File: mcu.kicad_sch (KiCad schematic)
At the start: 46 parts, among them CN100 HX JN1.27-2X5 TP H4.9, J100 DM3CS-SF, U100 SW_RUN, U101 STM32F405RGTx, X100 X1E000210127000G

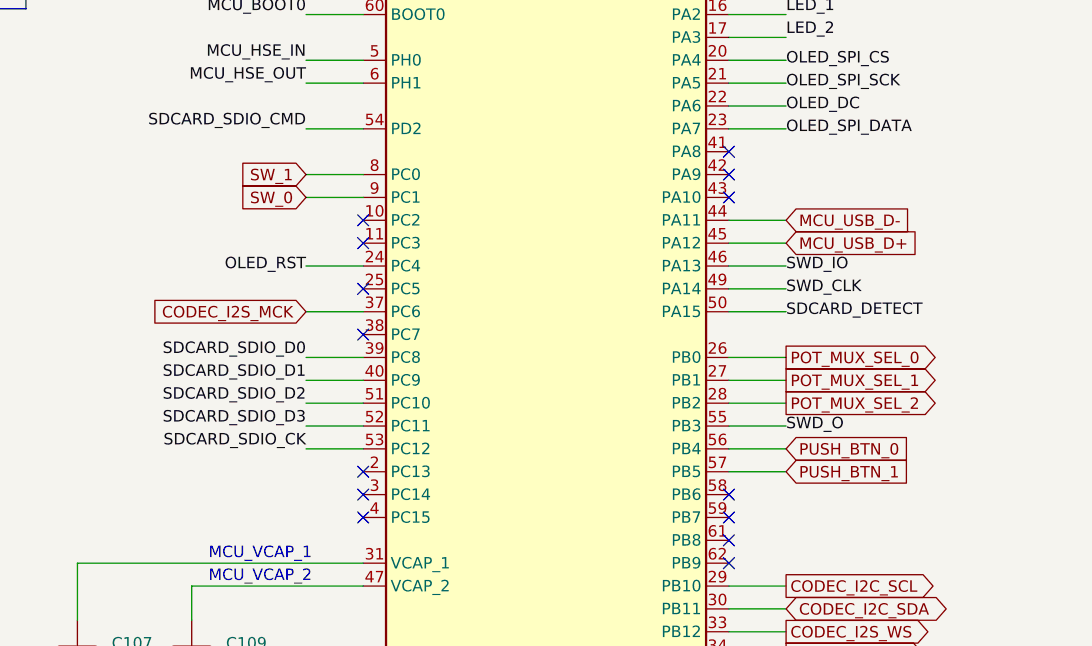
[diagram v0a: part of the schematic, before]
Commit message: last status
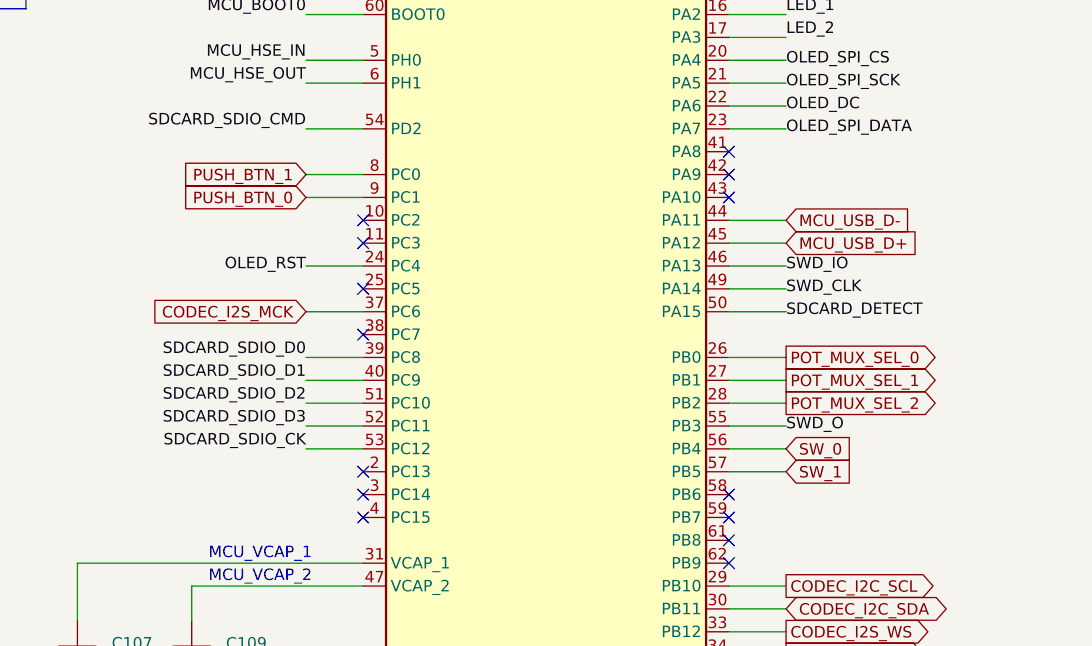
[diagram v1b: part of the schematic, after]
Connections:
- net PUSH_BTN_0: now also U101.9 (PC1); no longer U101.56 (PB4)
- net PUSH_BTN_1: now also U101.8 (PC0); no longer U101.57 (PB5)
- net SW_0: now also U101.56 (PB4); no longer U101.9 (PC1)
- net SW_1: now also U101.57 (PB5); no longer U101.8 (PC0)
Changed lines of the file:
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@@
 		)
 	)
-	(global_label "SW_1"
+	(global_label "PUSH_BTN_1"
 		(shape input)
 		(at 187.96 76.2 180)
@@
 		)
 		(property "Intersheetrefs" "${INTERSHEET_REFS}"
-			(at 180.1368 76.2 0)
+			(at 173.1215 76.2 0)
 			(effects
 				(font
@@
 		)
 	)
-	(global_label "PUSH_BTN_0"
+	(global_label "SW_0"
 		(shape input)
 		(at 241.3 106.68 0)
@@
 		)
 		(property "Intersheetrefs" "${INTERSHEET_REFS}"
-			(at 256.1385 106.68 0)
+			(at 249.1232 106.68 0)
 			(effects
 				(font
@@
 		)
 	)
-	(global_label "PUSH_BTN_1"
+	(global_label "SW_1"
 		(shape input)
 		(at 241.3 109.22 0)
@@
 		)
 		(property "Intersheetrefs" "${INTERSHEET_REFS}"
-			(at 256.1385 109.22 0)
+			(at 249.1232 109.22 0)
 			(effects
 				(font
@@
 		)
 	)
-	(global_label "SW_0"
+	(global_label "PUSH_BTN_0"
 		(shape input)
 		(at 187.96 78.74 180)
@@
 		)
 		(property "Intersheetrefs" "${INTERSHEET_REFS}"
-			(at 180.1368 78.74 0)
-			(effects
-				(font
+			(at 173.1215 78.74 0)
+			(effects
+				(font
